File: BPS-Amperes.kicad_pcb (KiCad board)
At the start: 2 copper layers, 40 x 35 mm, 52 parts, among them J1 ShuntConn, J2 LeaderConn, J3 Conn_01x04, J4 Conn_01x05, U1 INA186A3IDDFT, U2 RO-123.3S_HP, U3 LTC6820, U4 HX1188FNL, U5 REF1930AIDDCT, U6 LTC2315, U7 OPA2196

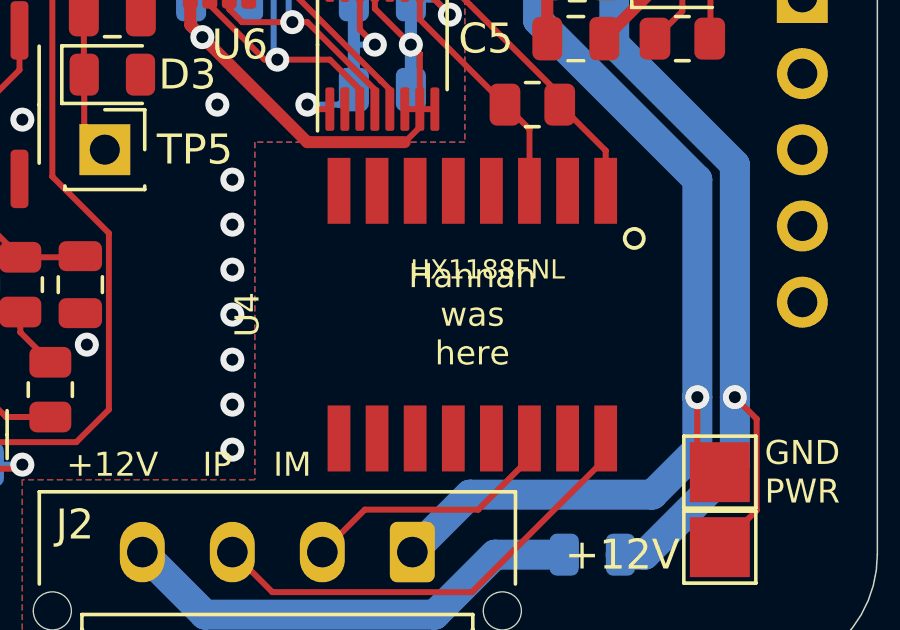
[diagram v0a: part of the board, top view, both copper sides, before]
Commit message: text
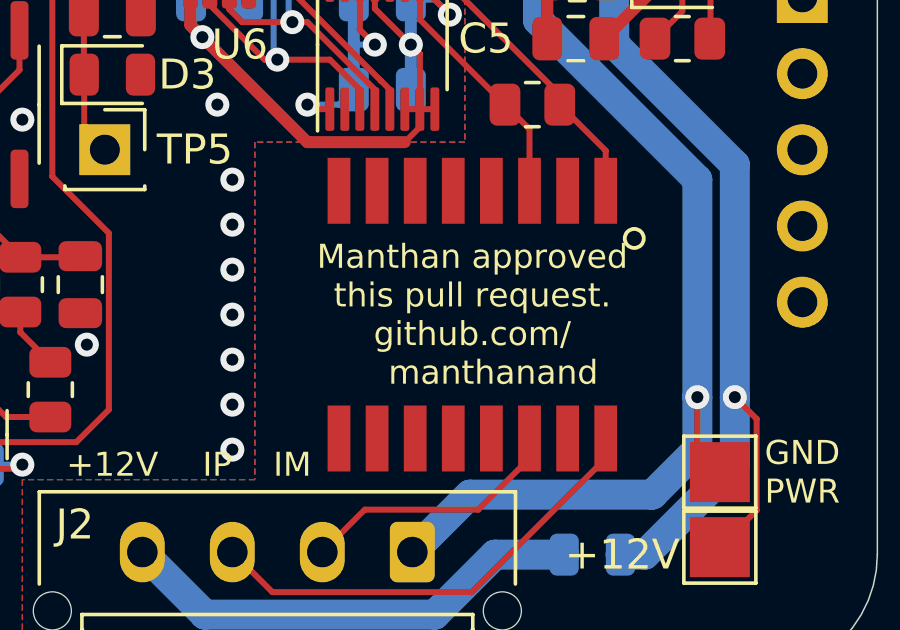
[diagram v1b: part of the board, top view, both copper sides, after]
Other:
- board text added: "Manthan approved this pull request. github.com/ manthanand"
- board text removed: "Hannah was here"
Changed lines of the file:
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@@
     (property "Sheetname" "")
     (attr smd)
-    (fp_text reference "U4" (at 7.5 0 90) (layer "F.SilkS")
+    (fp_text reference "U4" (at 7.5 0 90) (layer "F.SilkS") hide
       (effects (font (size 0.801614 0.801614) (thickness 0.05)))
     )
-    (fp_text value "HX1188FNL" (at -0.50895 1.50142) (layer "F.SilkS")
+    (fp_text value "HX1188FNL" (at -0.50895 1.50142) (layer "F.SilkS") hide
       (effects (font (size 0.641203 0.641203) (thickness 0.05)))
     )
@@
     (effects (font (size 0.8 0.8) (thickness 0.15)))
   )
-  (gr_text "Hannah\nwas\nhere" (at 141.5 118) (layer "F.SilkS")
+  (gr_text "Manthan approved\nthis pull request.\ngithub.com/\n	manthanand" (at 141.5 118) (layer "F.SilkS")
     (effects (font (size 0.8 0.8) (thickness 0.15)))
   )
